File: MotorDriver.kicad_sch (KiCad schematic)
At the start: 16 parts, among them J1 43045-0402, U28 DRV8462DDWR

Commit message: updated some part numbers
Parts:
- C38, C39, C9: Model CAP CER 10000PF 100V X7R 0805 -> CL21B103KCANNNC
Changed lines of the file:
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@@
       (effects (font (size 1.27 1.27)) hide)
     )
-    (property "Model" "CAP CER 10000PF 100V X7R 0805" (id 4) (at 167.005 87.63 0)
+    (property "Description" "CAP CER 10000PF 100V X7R 0805" (id 4) (at 167.005 87.63 0)
+      (effects (font (size 1.27 1.27)) hide)
+    )
+    (property "Model" "CL21B103KCANNNC" (id 5) (at 167.005 87.63 90)
       (effects (font (size 1.27 1.27)) hide)
     )
@@
       (effects (font (size 1.27 1.27)) hide)
     )
-    (property "Model" "CAP CER 10000PF 100V X7R 0805" (id 4) (at 167.64 109.22 0)
+    (property "Description" "CAP CER 10000PF 100V X7R 0805" (id 4) (at 167.64 109.22 0)
+      (effects (font (size 1.27 1.27)) hide)
+    )
+    (property "Model" "CL21B103KCANNNC" (id 5) (at 167.64 109.22 90)
       (effects (font (size 1.27 1.27)) hide)
     )
@@
       (effects (font (size 1.27 1.27)) hide)
     )
-    (property "Model" "CAP CER 10000PF 100V X7R 0805" (id 4) (at 166.37 63.5 0)
-      (effects (font (size 1.27 1.27)) hide)
-    )
+    (property "Description" "CAP CER 10000PF 100V X7R 0805" (id 4) (at 166.37 63.5 0)
+      (effects (font (size 1.27 1.27)) hide)
+    )
+    (property "Model" "CL21B103KCANNNC" (id 5) (at 166.37 63.5 90)
+      (effects (font (size 1.27 1.27)) hide)
+    )

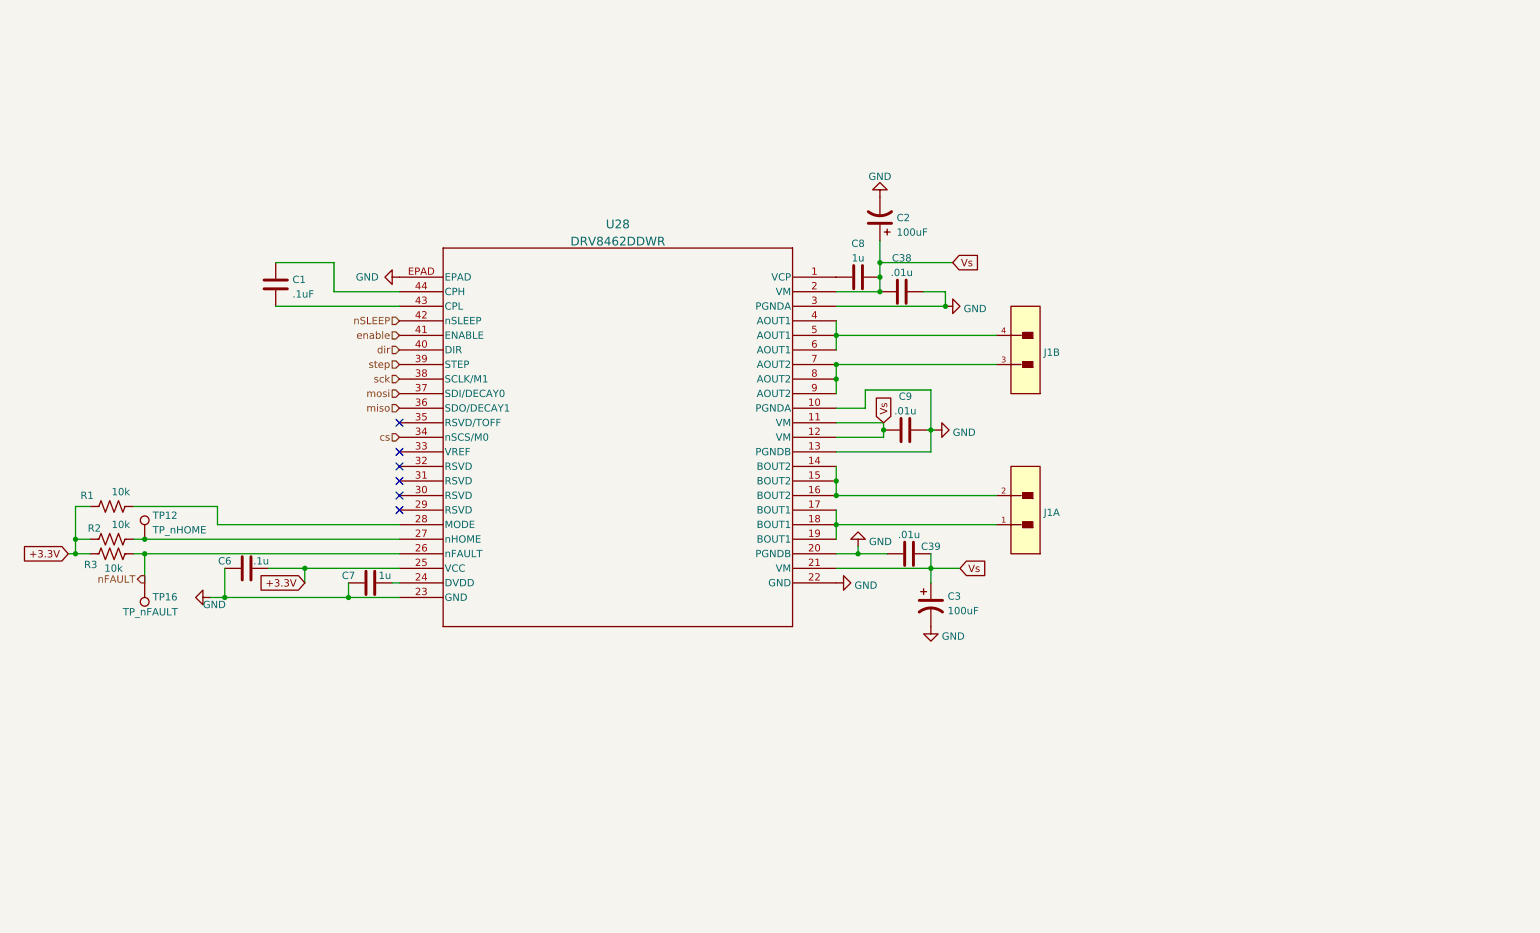
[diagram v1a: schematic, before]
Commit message: Move back to drv8711
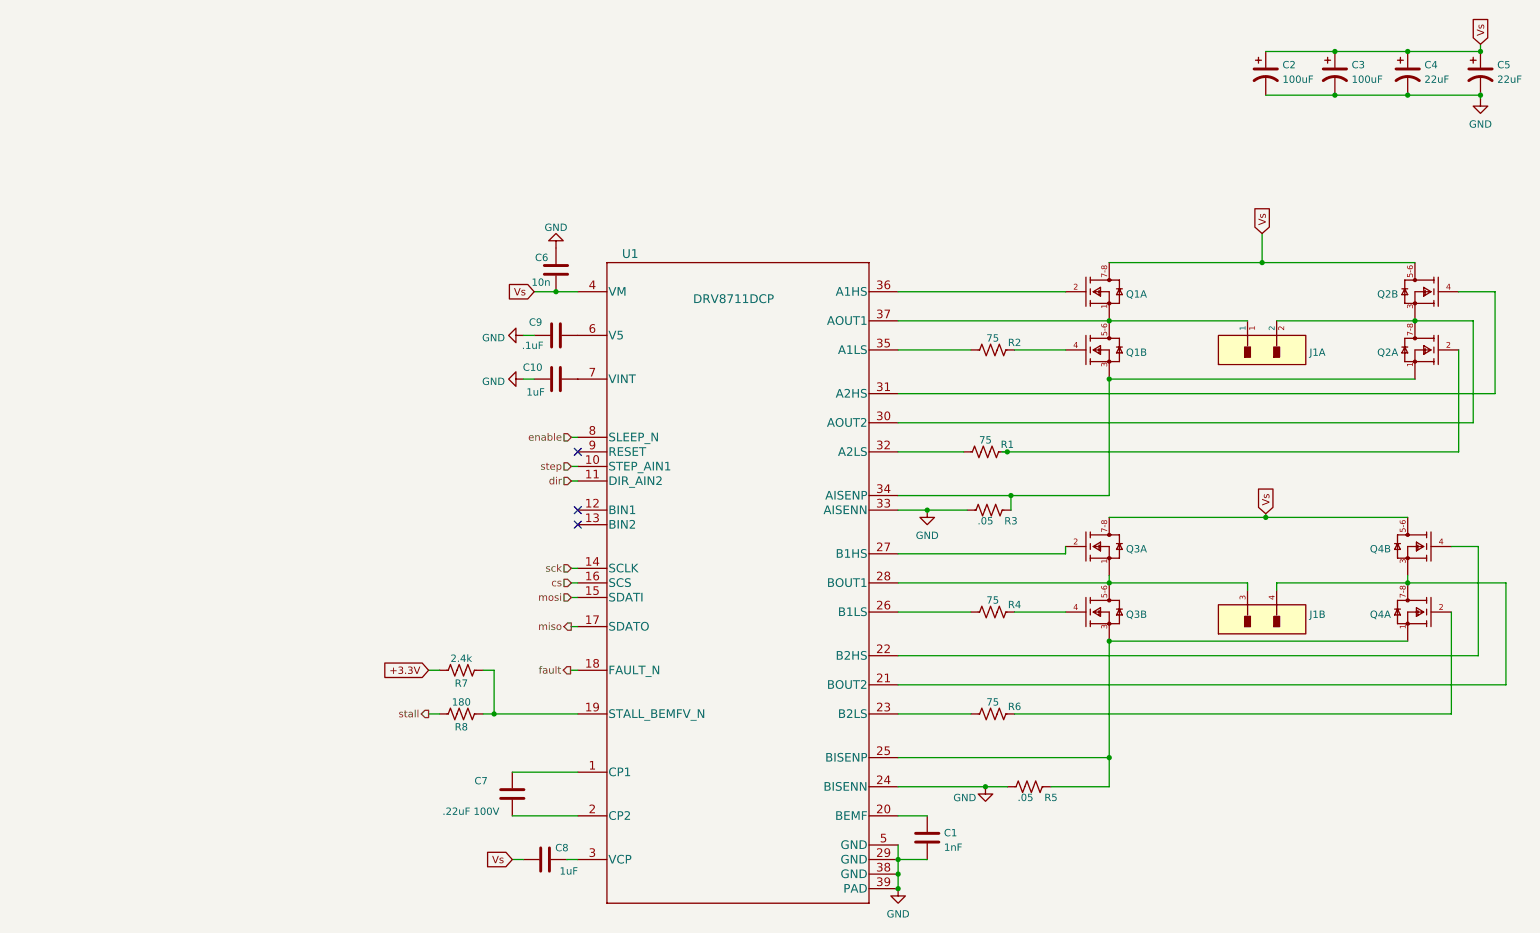
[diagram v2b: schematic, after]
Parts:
- removed C38, C39: .01u, Capacitor_SMD:C_0805_2012Metric_Pad1.18x1.45mm_HandSolder, symbol Device:C
- removed TP12: TP_nHOME, Project_Footprints_Library:test_point, symbol Connector:TestPoint
- removed TP16: TP_nFAULT, Project_Footprints_Library:test_point, symbol Connector:TestPoint
- removed U28: DRV8462DDWR, Project_Footprints_Library:DDW44_8P26X4P31, symbol 1LibBBCTRL:DRV8462DDWR
- added C10: 1uF, Capacitor_SMD:C_0805_2012Metric_Pad1.18x1.45mm_HandSolder, symbol Device:C
- added C4, C5: 22uF, Capacitor_THT:CP_Radial_D5.0mm_P2.00mm, symbol Device:C_Polarized_US
- added Q1, Q2, Q3, Q4: DMTH6010LPD-13, Project_Footprints_Library:ON_Semiconductor-506BT-02_2013-E-MFG, symbol 1LibBBCTRL:NVMFD5C672NLT1G
- added R4, R6: 75, Resistor_SMD:R_0805_2012Metric_Pad1.20x1.40mm_HandSolder, symbol Device:R_US
- added R5: .05, Resistor_SMD:R_2512_6332Metric_Pad1.40x3.35mm_HandSolder, symbol Device:R_US
- added R7: 2.4k, Resistor_SMD:R_0805_2012Metric_Pad1.20x1.40mm_HandSolder, symbol Device:R_US
- added R8: 180, Resistor_SMD:R_0805_2012Metric_Pad1.20x1.40mm_HandSolder, symbol Device:R_US
- added U1: DRV8711DCP, Project_Footprints_Library:DRV8711DCP, symbol 1LibBBCTRL:DRV8711DCP
- C1: value .1uF -> 1nF; Model CL21B104KCFNNNE -> C0805C102K4RACTU
- C6: value .1u -> 10n; Model 08056D104KAT2A -> C0805C103K1RAC7210
- C7: value 1u -> .22uF 100V; Model CC0805KKX5R5BB105 -> CL21B224KCFSNWE
- C8: value 1u -> 1uF; Model CL21B105KOFNNNE -> CC0805KKX7R7BB105
- C9: value .01u -> .1uF; Model CL21B103KCANNNC -> C0805C104M5RACTU
- R1, R2: value 10k -> 75; Model RC0805FR-0710KL -> RMCF0805JT75R0
- R3: value 10k -> .05; footprint Resistor_SMD:R_0805_2012Metric_Pad1.20x1.40mm_HandSolder -> Resistor_SMD:R_2512_6332Metric_Pad1.40x3.35mm_HandSolder; Model RC0805FR-0710KL -> CSRL3-0R05F8
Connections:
- net +3.3V: now also R7.1; no longer C6.2, R1.1, R2.1, R3.1
- net GND: now also C1.2, C9.1, R3.1, C10.1, C4.2, C5.2, R5.1, U1.24 (BISENN), U1.29 (GND), U1.33 (AISENN), U1.38 (GND), U1.39 (PAD), U1.5 (GND); no longer C7.1, C9.2
- net Vs: now also C6.2, C8.2, C4.1, C5.1, Q1.7-8 (D1), Q2.5-6 (D2), Q3.7-8 (D1), Q4.5-6 (D2), U1.4 (VM); no longer C8.1, C9.1
- net cs: now also U1.16 (SCS)
- net dir: now also U1.11 (DIR_AIN2)
- net enable: now also U1.8 (SLEEP_N)
- net miso: now also U1.17 (SDATO)
- net mosi: now also U1.15 (SDATI)
- net sck: now also U1.14 (SCLK)
- net step: now also U1.10 (STEP_AIN1)
- net at R2.2: now also Q1.4 (G2)
- net at J1.1: now also Q1.1 (S1), Q1.5-6 (D2), U1.37 (AOUT1)
- net at J1.2: now also Q2.3 (S2), Q2.7-8 (D1), U1.30 (AOUT2)
- net at C7.2: now also U1.2 (CP2)
- net at C1.1: now also U1.20 (BEMF)
- net at J1.3: now also Q3.1 (S1), Q3.5-6 (D2), U1.28 (BOUT1)
- net at J1.4: now also Q4.3 (S2), Q4.7-8 (D1), U1.21 (BOUT2)
- net at R1.2: now also Q2.2 (G1)
- net nFAULT: no longer names the net of R3.2
- net nFAULT: now also Q1.3 (S2), Q2.1 (S1), U1.34 (AISENP)
- new net: Q3.3 (S2), Q4.1 (S1), R5.2, U1.25 (BISENP)
- new net: R6.1, U1.23 (B2LS)
- new net: Q4.2 (G1), R6.2
- new net: C7.1, U1.1 (CP1)
- new net: C10.2, U1.7 (VINT)
- new net: R7.2, R8.2, U1.19 (STALL_BEMFV_N)
- new net: R2.1, U1.35 (A1LS)
- new net: Q3.2 (G1), U1.27 (B1HS)
- new net: Q3.4 (G2), R4.2
- new net: Q2.4 (G2), U1.31 (A2HS)
- new net: Q4.4 (G2), U1.22 (B2HS)
- new net: R4.1, U1.26 (B1LS)
- new net: C8.1, U1.3 (VCP)
- new net: R1.1, U1.32 (A2LS)
- new net: Q1.2 (G1), U1.36 (A1HS)
- new net: C9.2, U1.6 (V5)
- new net fault: U1.18 (FAULT_N)
- new net stall: R8.1
- no-connect marks 6 -> 3
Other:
- moved on the sheet: C2, C3, J1B
